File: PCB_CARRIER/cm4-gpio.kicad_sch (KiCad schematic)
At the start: 28 parts, among them Q1 BSS138, Q2 BSS138, Q3 BSS138

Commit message: going to school now
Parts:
- SW?: footprint (none) -> Button_Switch_THT:SW_DIP_SPSTx04_Slide_6.7x11.72mm_W7.62mm_P2.54mm_LowProfile
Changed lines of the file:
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@@
 		(on_board yes)
 		(dnp no)
-		(property "Reference" "#PWR?"
+		(property "Reference" "#PWR0102"
 			(at 102.87 165.1 0)
 			(effects
@@
 			(project "carrier"
 				(path "/f52509e6-8053-454c-b8e9-3e2670c5a5fe/fc4c71a5-1008-4ac4-98db-57c838c57d91"
-					(reference "#PWR?")
+					(reference "#PWR0102")
 					(unit 1)
 				)
@@
 		(on_board yes)
 		(dnp no)
-		(property "Reference" "#PWR?"
+		(property "Reference" "#PWR0105"
 			(at 100.33 139.7 0)
 			(effects
@@
 			(project "carrier"
 				(path "/f52509e6-8053-454c-b8e9-3e2670c5a5fe/fc4c71a5-1008-4ac4-98db-57c838c57d91"
-					(reference "#PWR?")
+					(reference "#PWR0105")
 					(unit 1)
 				)
@@
 		(dnp no)
 		(fields_autoplaced yes)
-		(property "Reference" "#PWR?"
+		(property "Reference" "#PWR0101"
 			(at 58.42 95.25 0)
 			(effects
@@
 			(project "carrier"
 				(path "/f52509e6-8053-454c-b8e9-3e2670c5a5fe/fc4c71a5-1008-4ac4-98db-57c838c57d91"
-					(reference "#PWR?")
+					(reference "#PWR0101")
 					(unit 1)
 				)
@@
 		(dnp no)
 		(fields_autoplaced yes)
-		(property "Reference" "#PWR?"
+		(property "Reference" "#PWR0114"
 			(at 265.43 180.34 0)
 			(effects
@@
 			(project "carrier"
 				(path "/f52509e6-8053-454c-b8e9-3e2670c5a5fe/fc4c71a5-1008-4ac4-98db-57c838c57d91"
-					(reference "#PWR?")
+					(reference "#PWR0114")
 					(unit 1)
 				)
@@
 		(on_board yes)
 		(dnp no)
-		(property "Reference" "#PWR?"
+		(property "Reference" "#PWR0113"
 			(at 168.91 165.1 0)
 			(effects
@@
 			(project "carrier"
 				(path "/f52509e6-8053-454c-b8e9-3e2670c5a5fe/fc4c71a5-1008-4ac4-98db-57c838c57d91"
-					(reference "#PWR?")
+					(reference "#PWR0113")
 					(unit 1)
 				)
@@
 		(dnp no)
 		(fields_autoplaced yes)
-		(property "Reference" "#PWR?"
+		(property "Reference" "#PWR0107"
 			(at 276.86 91.44 0)
 			(effects
@@
 			(project "carrier"
 				(path "/f52509e6-8053-454c-b8e9-3e2670c5a5fe/fc4c71a5-1008-4ac4-98db-57c838c57d91"
-					(reference "#PWR?")
+					(reference "#PWR0107")
 					(unit 1)
 				)
@@
 		(dnp no)
 		(fields_autoplaced yes)
-		(property "Reference" "#PWR?"
+		(property "Reference" "#PWR0112"
 			(at 246.38 127 0)
 			(effects
@@
 			(project "carrier"
 				(path "/f52509e6-8053-454c-b8e9-3e2670c5a5fe/fc4c71a5-1008-4ac4-98db-57c838c57d91"
-					(reference "#PWR?")
+					(reference "#PWR0112")
 					(unit 1)
 				)
@@
 		(on_board yes)
 		(dnp no)
-		(property "Reference" "#PWR?"
+		(property "Reference" "#PWR0111"
 			(at 215.9 139.7 0)
 			(effects
@@
 			(project "carrier"
 				(path "/f52509e6-8053-454c-b8e9-3e2670c5a5fe/fc4c71a5-1008-4ac4-98db-57c838c57d91"
-					(reference "#PWR?")
+					(reference "#PWR0111")
 					(unit 1)
 				)
@@
 		(on_board yes)
 		(dnp no)
-		(property "Reference" "#PWR?"
+		(property "Reference" "#PWR0106"
 			(at 100.33 144.78 0)
 			(effects
@@
 			(project "carrier"
 				(path "/f52509e6-8053-454c-b8e9-3e2670c5a5fe/fc4c71a5-1008-4ac4-98db-57c838c57d91"
-					(reference "#PWR?")
+					(reference "#PWR0106")
 					(unit 1)
 				)
@@
 			)
 		)
-		(property "Footprint" ""
+		(property "Footprint" "Button_Switch_THT:SW_DIP_SPSTx04_Slide_6.7x11.72mm_W7.62mm_P2.54mm_LowProfile"
 			(at 254 113.03 0)
 			(effects
@@
 		(on_board yes)
 		(dnp no)
-		(property "Reference" "#PWR?"
+		(property "Reference" "#PWR0110"
 			(at 215.9 129.54 0)
 			(effects
@@
 			(project "carrier"
 				(path "/f52509e6-8053-454c-b8e9-3e2670c5a5fe/fc4c71a5-1008-4ac4-98db-57c838c57d91"
-					(reference "#PWR?")
+					(reference "#PWR0110")
 					(unit 1)
 				)
@@
 		(dnp no)
 		(fields_autoplaced yes)
-		(property "Reference" "#PWR?"
+		(property "Reference" "#PWR0109"
 			(at 237.49 29.21 0)
 			(effects
@@
 			(project "carrier"
 				(path "/f52509e6-8053-454c-b8e9-3e2670c5a5fe/fc4c71a5-1008-4ac4-98db-57c838c57d91"
-					(reference "#PWR?")
+					(reference "#PWR0109")
 					(unit 1)
 				)
@@
 		(dnp no)
 		(fields_autoplaced yes)
-		(property "Reference" "#PWR?"
+		(property "Reference" "#PWR0108"
 			(at 255.27 45.72 0)
 			(effects
@@
 			(project "carrier"
 				(path "/f52509e6-8053-454c-b8e9-3e2670c5a5fe/fc4c71a5-1008-4ac4-98db-57c838c57d91"
-					(reference "#PWR?")
+					(reference "#PWR0108")
 					(unit 1)
 				)

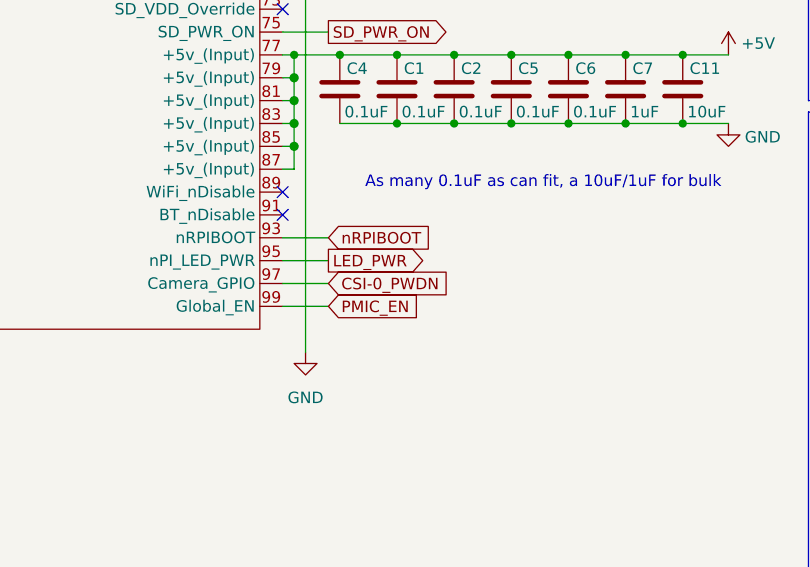
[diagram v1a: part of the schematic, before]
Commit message: fixed camera power pins, oops, researching a lot about level shifting
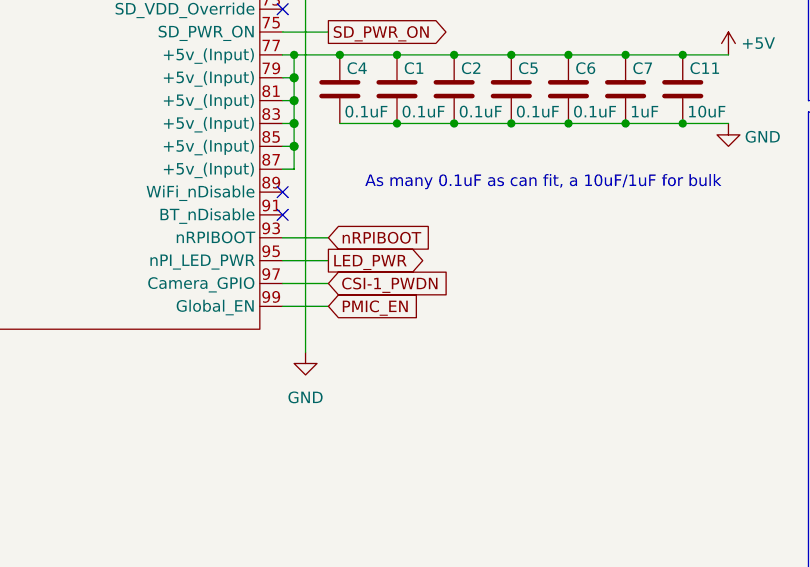
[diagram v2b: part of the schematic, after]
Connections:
- net CSI-0_PWDN: no longer Module?.97 (Camera_GPIO)
- new net CSI-1_PWDN: Module?.97 (Camera_GPIO)
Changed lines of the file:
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@@
 		)
 	)
-	(global_label "CSI-0_PWDN"
+	(global_label "CSI-1_PWDN"
 		(shape input)
 		(at 171.45 151.13 0)

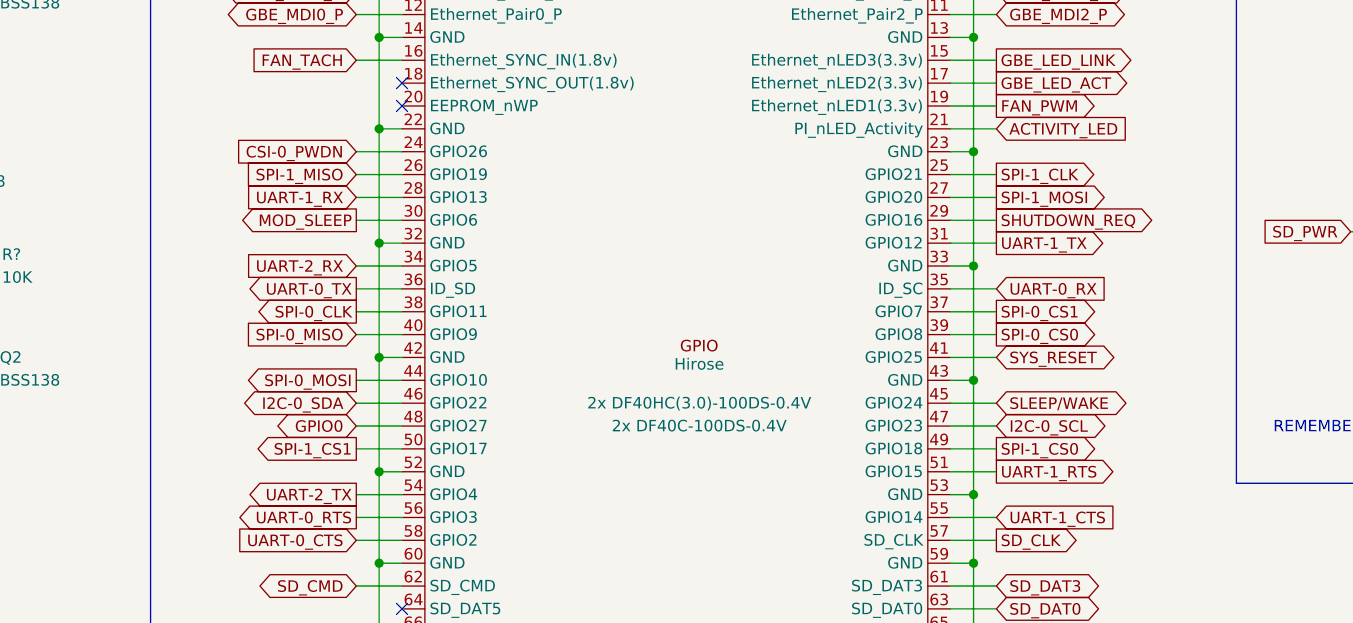
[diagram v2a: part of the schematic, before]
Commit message: SPI inputs to level shift
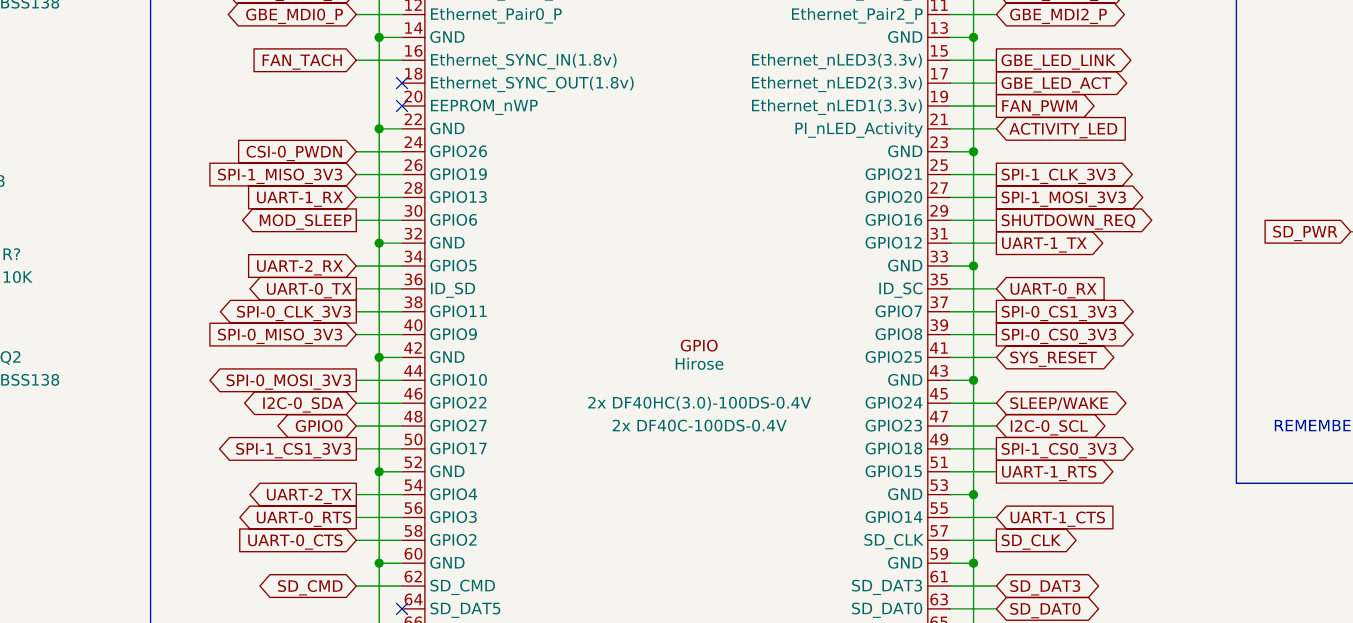
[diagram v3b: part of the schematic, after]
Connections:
- net SPI-0_CLK renamed SPI-0_CLK_3V3
- net SPI-0_CS0 renamed SPI-0_CS0_3V3
- net SPI-0_CS1 renamed SPI-0_CS1_3V3
- net SPI-0_MISO renamed SPI-0_MISO_3V3
- net SPI-0_MOSI renamed SPI-0_MOSI_3V3
- net SPI-1_CLK renamed SPI-1_CLK_3V3
- net SPI-1_CS0 renamed SPI-1_CS0_3V3
- net SPI-1_CS1 renamed SPI-1_CS1_3V3
- net SPI-1_MISO renamed SPI-1_MISO_3V3
- net SPI-1_MOSI renamed SPI-1_MOSI_3V3
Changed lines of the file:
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@@
 		)
 	)
-	(global_label "SPI-1_MISO"
+	(global_label "SPI-1_MISO_3V3"
 		(shape input)
 		(at 100.33 59.69 180)
@@
 		)
 		(property "Intersheetrefs" "${INTERSHEET_REFS}"
-			(at 85.8197 59.69 0)
+			(at 81.3445 59.69 0)
 			(effects
 				(font
@@
 		)
 	)
-	(global_label "SPI-1_CLK"
+	(global_label "SPI-1_CLK_3V3"
 		(shape output)
 		(at 171.45 59.69 0)
@@
 		)
 		(property "Intersheetrefs" "${INTERSHEET_REFS}"
-			(at 184.9322 59.69 0)
+			(at 189.4074 59.69 0)
 			(effects
 				(font
@@
 		)
 	)
-	(global_label "SPI-1_CS1"
+	(global_label "SPI-1_CS1_3V3"
 		(shape output)
 		(at 100.33 90.17 180)
@@
 		)
 		(property "Intersheetrefs" "${INTERSHEET_REFS}"
-			(at 86.7269 90.17 0)
+			(at 82.2517 90.17 0)
 			(effects
 				(font
@@
 		)
 	)
-	(global_label "SPI-0_CS1"
+	(global_label "SPI-0_CS1_3V3"
 		(shape output)
 		(at 171.45 74.93 0)
@@
 		)
 		(property "Intersheetrefs" "${INTERSHEET_REFS}"
-			(at 185.0531 74.93 0)
+			(at 189.5283 74.93 0)
 			(effects
 				(font
@@
 		)
 	)
-	(global_label "SPI-1_MOSI"
+	(global_label "SPI-1_MOSI_3V3"
 		(shape output)
 		(at 171.45 62.23 0)
@@
 		)
 		(property "Intersheetrefs" "${INTERSHEET_REFS}"
-			(at 185.9603 62.23 0)
+			(at 190.4355 62.23 0)
 			(effects
 				(font
@@
 		)
 	)
-	(global_label "SPI-1_CS0"
+	(global_label "SPI-1_CS0_3V3"
 		(shape output)
 		(at 171.45 90.17 0)
@@
 		)
 		(property "Intersheetrefs" "${INTERSHEET_REFS}"
-			(at 185.0531 90.17 0)
+			(at 189.5283 90.17 0)
 			(effects
 				(font
@@
 		)
 	)
-	(global_label "SPI-0_MOSI"
+	(global_label "SPI-0_MOSI_3V3"
 		(shape output)
 		(at 100.33 82.55 180)
@@
 		)
 		(property "Intersheetrefs" "${INTERSHEET_REFS}"
-			(at 85.8197 82.55 0)
-			(effects
-				(font
-					(size 1.27 1.27)
-				)
-				(justify right)
-				(hide yes)
-			)
-		)
-	)
-	(global_label "SPI-0_CS0"
+			(at 81.3445 82.55 0)
+			(effects
+				(font
+					(size 1.27 1.27)
+				)
+				(justify right)
+				(hide yes)
+			)
+		)
+	)
+	(global_label "SPI-0_CS0_3V3"
 		(shape output)
 		(at 171.45 77.47 0)
@@
 		)
 		(property "Intersheetrefs" "${INTERSHEET_REFS}"
-			(at 185.0531 77.47 0)
+			(at 189.5283 77.47 0)
 			(effects
 				(font
@@
 		)
 	)
-	(global_label "SPI-0_MISO"
+	(global_label "SPI-0_MISO_3V3"
 		(shape input)
 		(at 100.33 77.47 180)
@@
 		)
 		(property "Intersheetrefs" "${INTERSHEET_REFS}"
-			(at 85.8197 77.47 0)
+			(at 81.3445 77.47 0)
 			(effects
 				(font
@@
 		)
 	)
-	(global_label "SPI-0_CLK"
+	(global_label "SPI-0_CLK_3V3"
 		(shape output)
 		(at 100.33 74.93 180)
@@
 		)
 		(property "Intersheetrefs" "${INTERSHEET_REFS}"
-			(at 86.8478 74.93 0)
-			(effects
-				(font
+			(at 82.3726 74.93 0)
+			(effects
+				(font

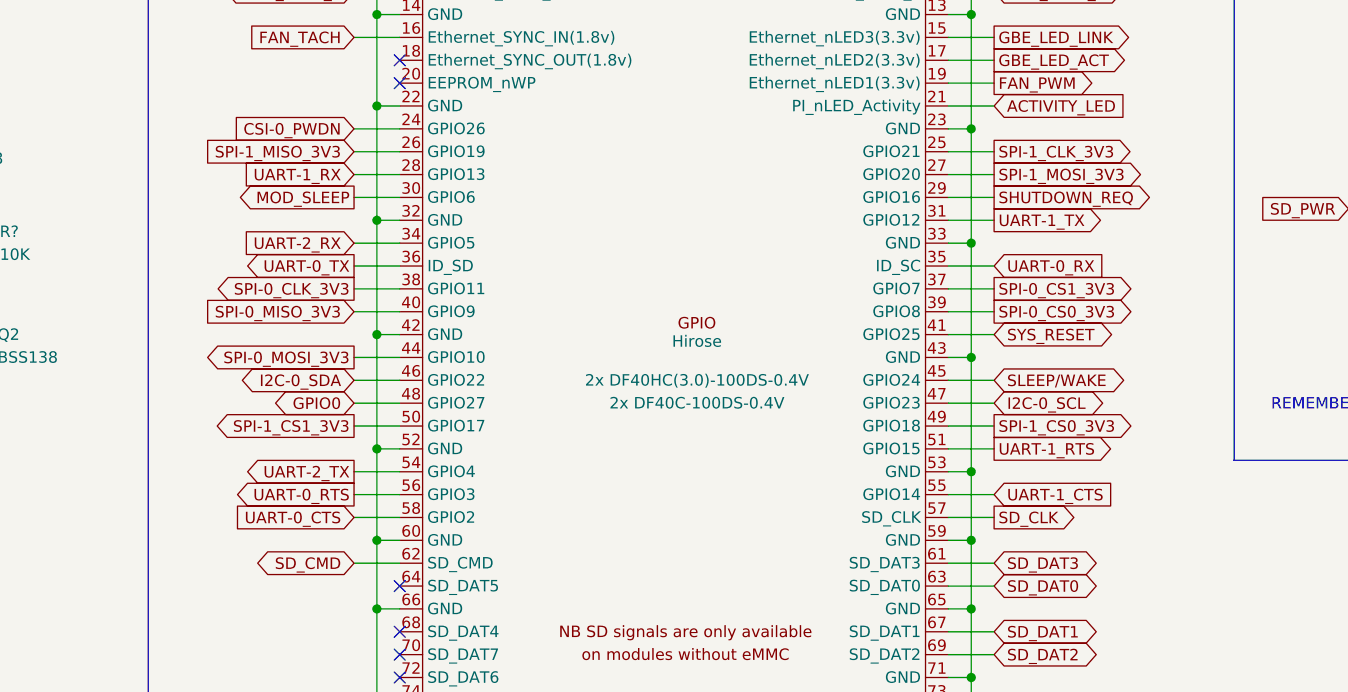
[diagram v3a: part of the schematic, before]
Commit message: re-naming all UART signals for shifting preparation
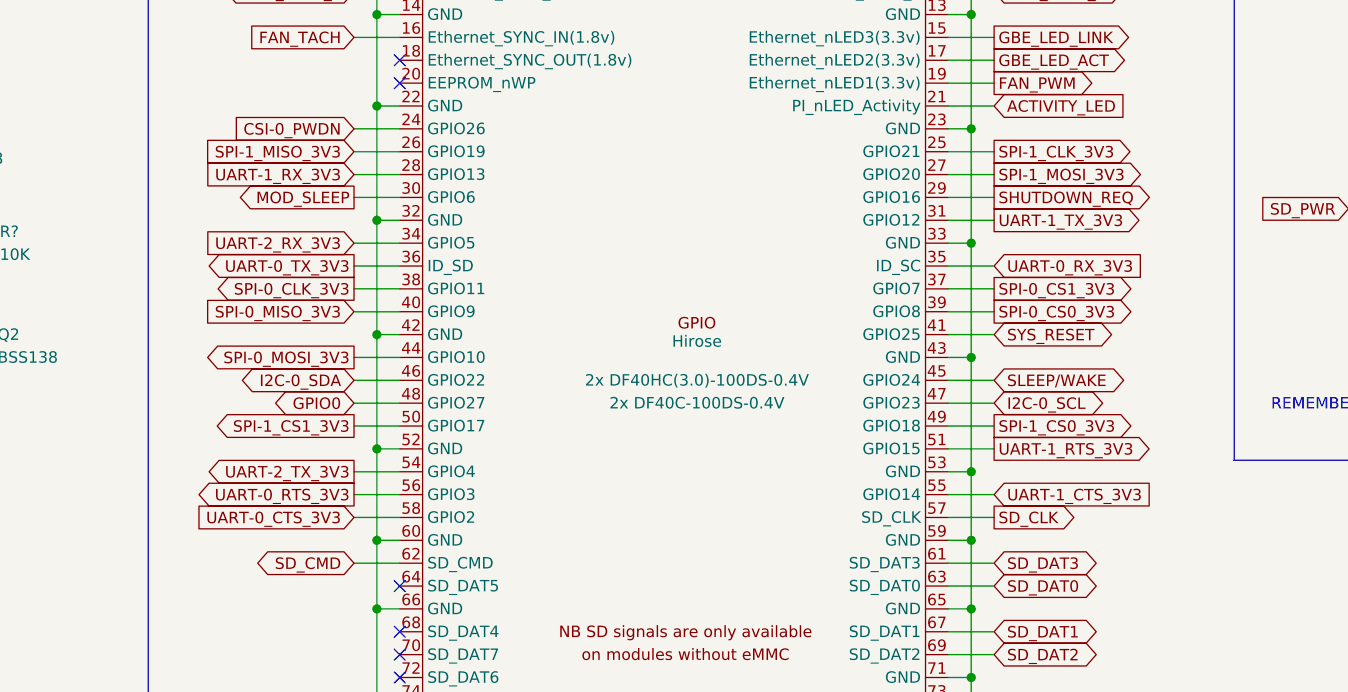
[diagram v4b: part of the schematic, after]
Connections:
- net UART-0_CTS renamed UART-0_CTS_3V3
- net UART-0_RTS renamed UART-0_RTS_3V3
- net UART-0_RX renamed UART-0_RX_3V3
- net UART-0_TX renamed UART-0_TX_3V3
- net UART-1_CTS renamed UART-1_CTS_3V3
- net UART-1_RTS renamed UART-1_RTS_3V3
- net UART-1_RX renamed UART-1_RX_3V3
- net UART-1_TX renamed UART-1_TX_3V3
- net UART-2_RX renamed UART-2_RX_3V3
- net UART-2_TX renamed UART-2_TX_3V3
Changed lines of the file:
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@@
 		)
 	)
-	(global_label "UART-1_TX"
+	(global_label "UART-1_TX_3V3"
 		(shape output)
 		(at 171.45 67.31 0)
@@
 		)
 		(property "Intersheetrefs" "${INTERSHEET_REFS}"
-			(at 185.1136 67.31 0)
-			(effects
-				(font
-					(size 1.27 1.27)
-				)
-				(justify left)
-				(hide yes)
-			)
-		)
-	)
-	(global_label "UART-2_TX"
+			(at 189.5888 67.31 0)
+			(effects
+				(font
+					(size 1.27 1.27)
+				)
+				(justify left)
+				(hide yes)
+			)
+		)
+	)
+	(global_label "UART-2_TX_3V3"
 		(shape output)
 		(at 100.33 95.25 180)
@@
 		)
 		(property "Intersheetrefs" "${INTERSHEET_REFS}"
-			(at 86.6664 95.25 0)
+			(at 82.1912 95.25 0)
 			(effects
 				(font
@@
 		)
 	)
-	(global_label "UART-0_TX"
+	(global_label "UART-0_TX_3V3"
 		(shape output)
 		(at 100.33 72.39 180)
@@
 		)
 		(property "Intersheetrefs" "${INTERSHEET_REFS}"
-			(at 86.6664 72.39 0)
+			(at 82.1912 72.39 0)
 			(effects
 				(font
@@
 		)
 	)
-	(global_label "UART-1_RTS"
+	(global_label "UART-1_RTS_3V3"
 		(shape output)
 		(at 171.45 92.71 0)
@@
 		)
 		(property "Intersheetrefs" "${INTERSHEET_REFS}"
-			(at 186.3836 92.71 0)
+			(at 190.8588 92.71 0)
 			(effects
 				(font
@@
 		)
 	)
-	(global_label "UART-0_RX"
+	(global_label "UART-0_RX_3V3"
 		(shape input)
 		(at 171.45 72.39 0)
@@
 		)
 		(property "Intersheetrefs" "${INTERSHEET_REFS}"
-			(at 185.416 72.39 0)
+			(at 189.8912 72.39 0)
 			(effects
 				(font
@@
 		)
 	)
-	(global_label "UART-0_CTS"
+	(global_label "UART-0_CTS_3V3"
 		(shape input)
 		(at 100.33 100.33 180)
@@
 		)
 		(property "Intersheetrefs" "${INTERSHEET_REFS}"
-			(at 85.3964 100.33 0)
+			(at 80.9212 100.33 0)
 			(effects
 				(font
@@
 		)
 	)
-	(global_label "UART-1_RX"
+	(global_label "UART-1_RX_3V3"
 		(shape input)
 		(at 100.33 62.23 180)
@@
 		)
 		(property "Intersheetrefs" "${INTERSHEET_REFS}"
-			(at 86.364 62.23 0)
-			(effects
-				(font
-					(size 1.27 1.27)
-				)
-				(justify right)
-				(hide yes)
-			)
-		)
-	)
-	(global_label "UART-2_RX"
+			(at 81.8888 62.23 0)
+			(effects
+				(font
+					(size 1.27 1.27)
+				)
+				(justify right)
+				(hide yes)
+			)
+		)
+	)
+	(global_label "UART-2_RX_3V3"
 		(shape input)
 		(at 100.33 69.85 180)
@@
 		)
 		(property "Intersheetrefs" "${INTERSHEET_REFS}"
-			(at 86.364 69.85 0)
+			(at 81.8888 69.85 0)
 			(effects
 				(font
@@
 		)
 	)
-	(global_label "UART-0_RTS"
+	(global_label "UART-0_RTS_3V3"
 		(shape output)
 		(at 100.33 97.79 180)
@@
 		)
 		(property "Intersheetrefs" "${INTERSHEET_REFS}"
-			(at 85.3964 97.79 0)
+			(at 80.9212 97.79 0)
 			(effects
 				(font
@@
 		)
 	)
-	(global_label "UART-1_CTS"
+	(global_label "UART-1_CTS_3V3"
 		(shape input)
 		(at 171.45 97.79 0)
@@
 		)
 		(property "Intersheetrefs" "${INTERSHEET_REFS}"
-			(at 186.3836 97.79 0)
-			(effects
-				(font
+			(at 190.8588 97.79 0)
+			(effects
+				(font
